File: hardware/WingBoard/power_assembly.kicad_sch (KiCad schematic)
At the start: 17 parts, among them J201 PWR_SEL, J202 Vin, SW201 SW_POWER, U201 AZ1117-5.0, U202 AZ1117-3.3

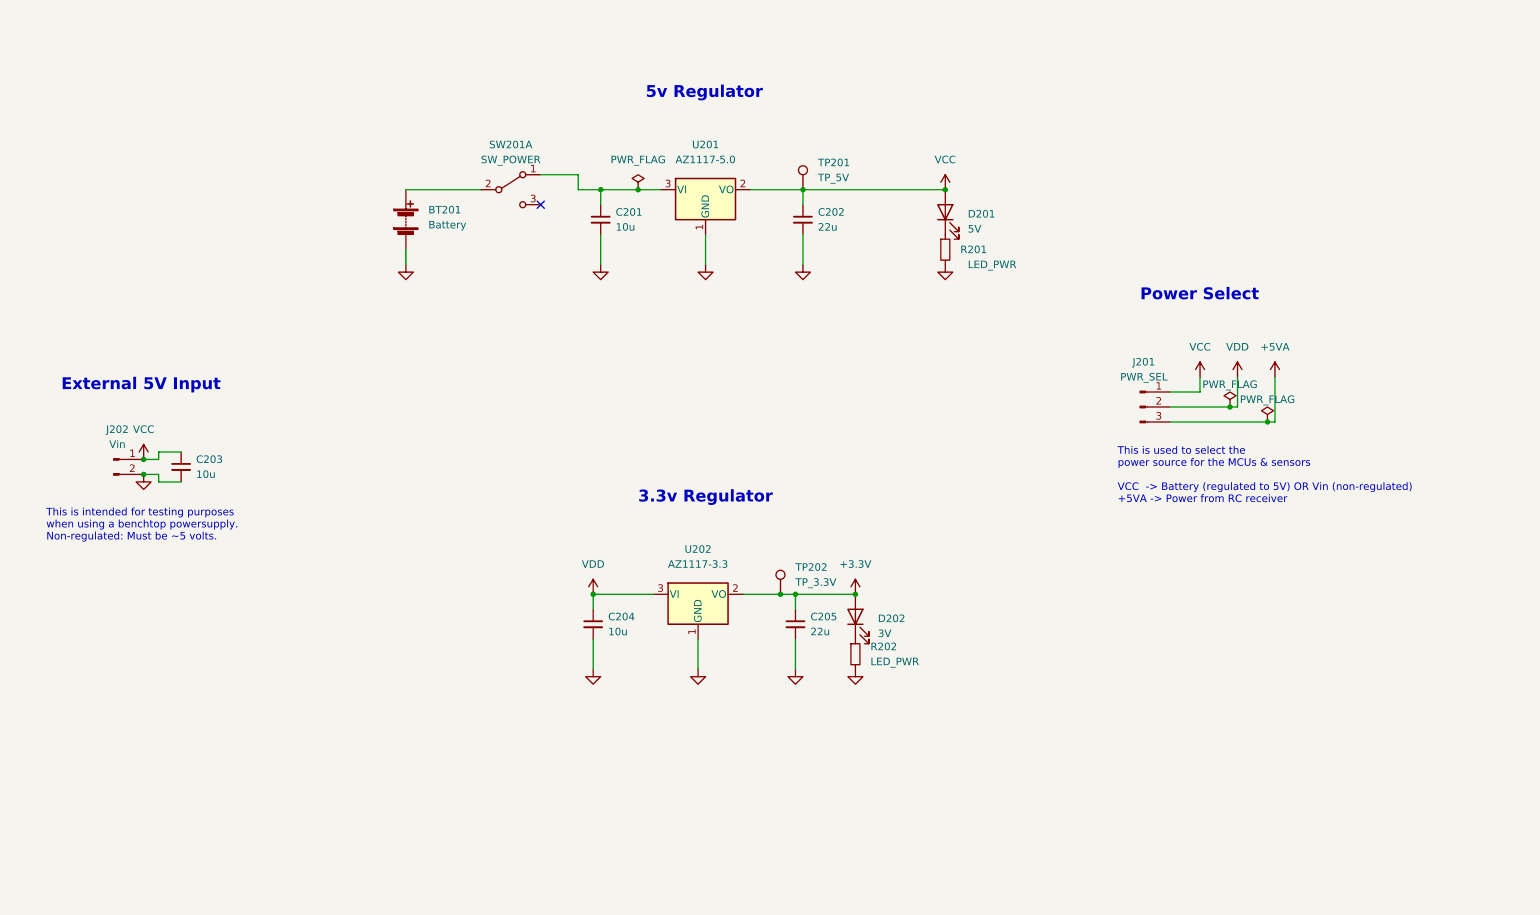
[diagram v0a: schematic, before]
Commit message: Hardware layout v0.1 complete.
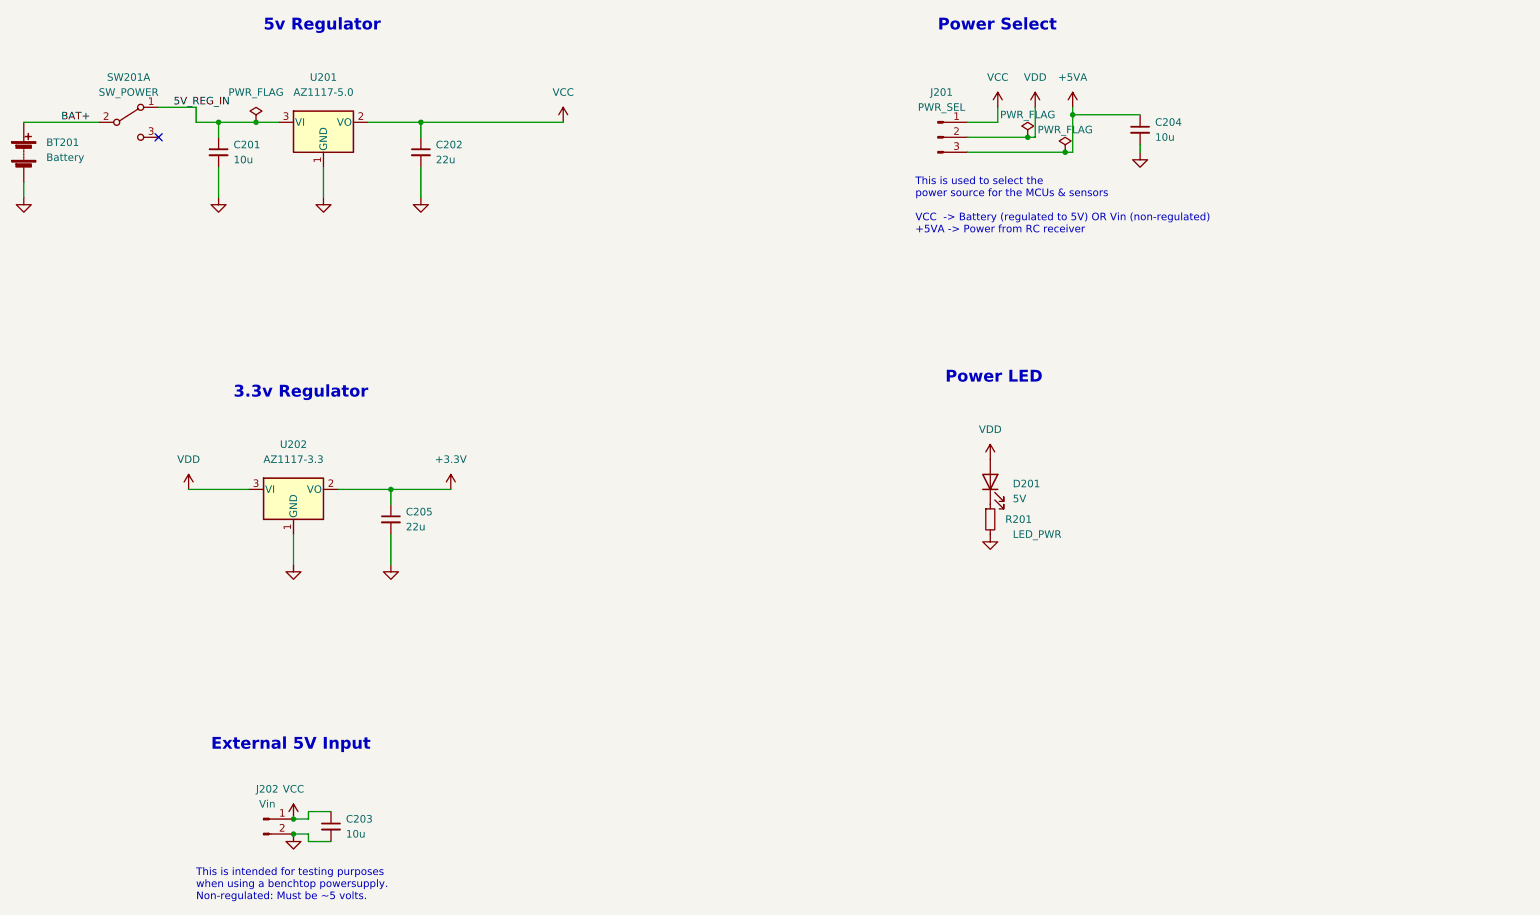
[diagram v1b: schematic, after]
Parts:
- removed D202: 3V, LED_SMD:LED_0805_2012Metric_Pad1.15x1.40mm_HandSolder, symbol Device:LED
- removed R202: LED_PWR, Resistor_SMD:R_0805_2012Metric_Pad1.20x1.40mm_HandSolder, symbol Device:R_Small
- removed TP201: TP_5V, TestPoint:TestPoint_Pad_D1.5mm, symbol Connector:TestPoint
- removed TP202: TP_3.3V, TestPoint:TestPoint_Pad_D1.5mm, symbol Connector:TestPoint
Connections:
- net +5VA: now also C204.1
- net VCC: no longer D201.2 (A)
- net VDD: now also D201.2 (A); no longer C204.1
- net 5V_REG_IN: now reaches C201.1, SW201.1 (A), U201.3 (VI)
- net BAT+: now reaches BT201.1 (+), SW201.2 (B)
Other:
- note added: "Power LED"
- moved on the sheet: BT201, C201, C202, C203, C205, D201, J201, J202, R201, SW201A, U201, U202
